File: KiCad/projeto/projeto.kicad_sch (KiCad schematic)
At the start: 21 parts, among them J2 HW-061, M1 Motor_Servo, M2 Motor_Servo, SW1 SW_Push, U1 HW-123E, U2 HC-SR04, U3 ESP-01S, U4 LM2596S-3.3, U5 LM2596S-5, U6 LM2596S-5, U7 LM2596S-5

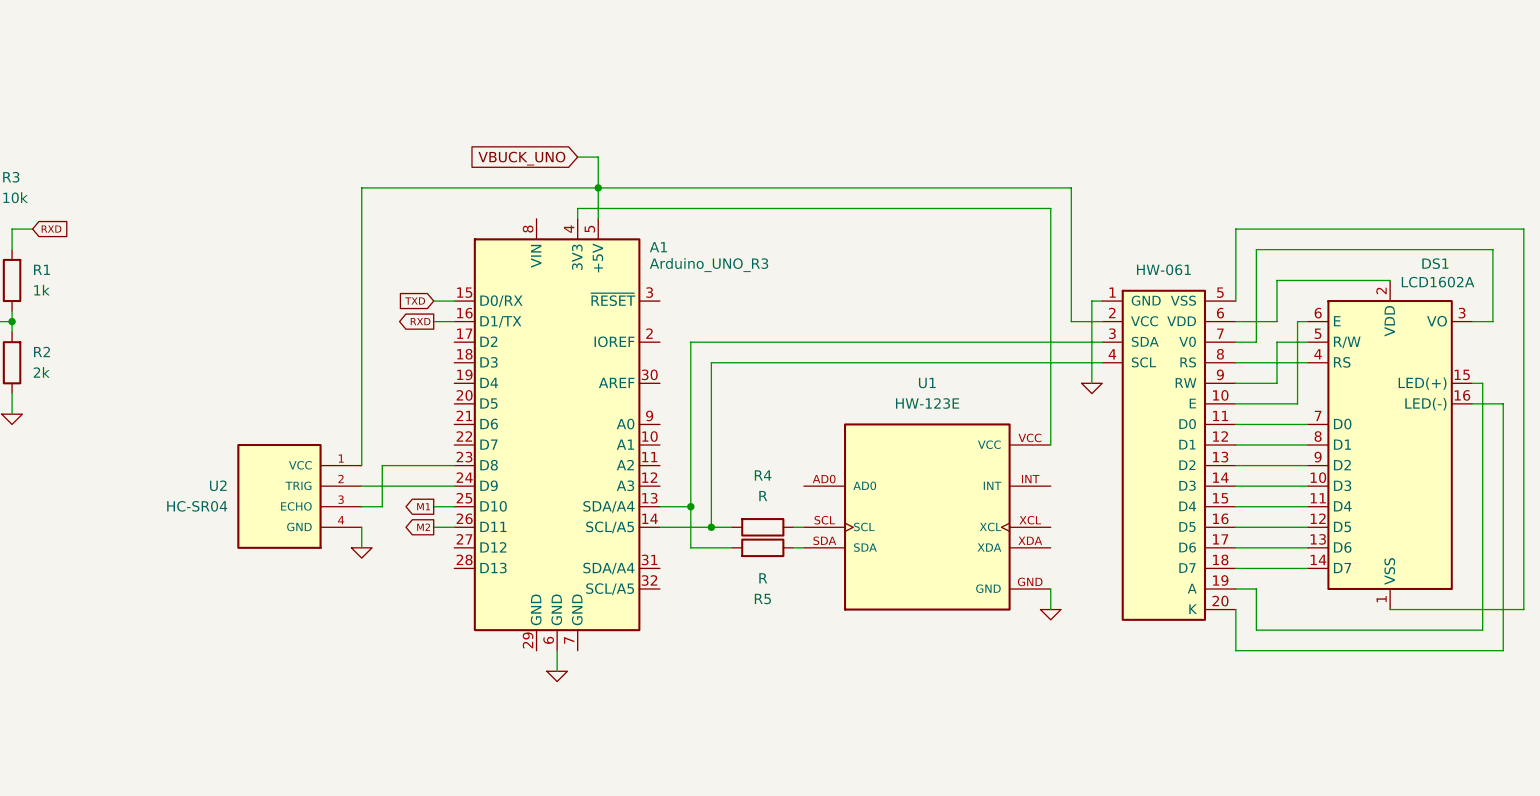
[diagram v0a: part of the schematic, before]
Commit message: Add files via upload
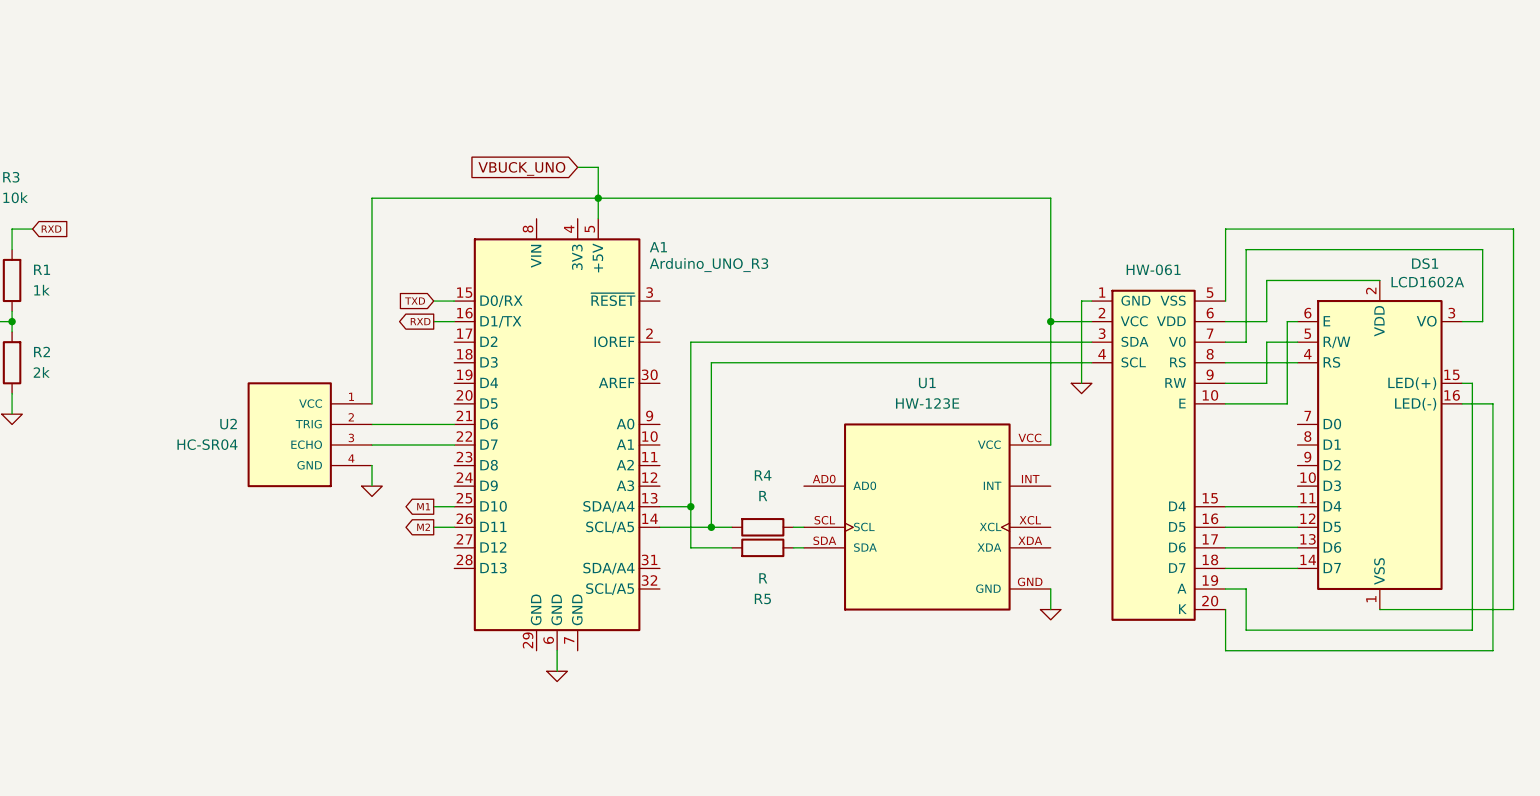
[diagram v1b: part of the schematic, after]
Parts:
- removed J2: HW-061, symbol Connector_Generic:Conn_01x16
- added J1: HW-061, symbol Connector_Generic:Conn_01x16
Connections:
- net 0: now also J1.1 (GND)
- net VBUCK_UNO: now also U1.VCC, J1.2 (VCC)
- net at DS1.6 (E): now also J1.10 (E)
- net at DS1.11 (D4): now also J1.15 (D4)
- net at DS1.12 (D5): now also J1.16 (D5)
- net at DS1.13 (D6): now also J1.17 (D6)
- net at DS1.14 (D7): now also J1.18 (D7)
- net at DS1.15 (LED(+)): now also J1.19 (A)
- net at DS1.16 (LED(-)): now also J1.20 (K)
- net at A1.13 (SDA/A4), R5.2: now also J1.3 (SDA)
- net at A1.14 (SCL/A5), R4.2: now also J1.4 (SCL)
- net at DS1.1 (VSS): now also J1.5 (VSS)
- net at DS1.2 (VDD): now also J1.6 (VDD)
- net at DS1.3 (VO): now also J1.7 (V0)
- net at DS1.4 (RS): now also J1.8 (RS)
- net at DS1.5 (R/W): now also J1.9 (RW)
- net at U2.2 (TRIG): now also A1.21 (D6); no longer A1.24 (D9)
- net at U2.3 (ECHO): now also A1.22 (D7); no longer A1.23 (D8)
- net at A1.4 (3V3): no longer U1.VCC
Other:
- moved on the sheet: DS1, U2
